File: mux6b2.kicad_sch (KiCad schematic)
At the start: 7 parts, among them U1 4081, U10 4071, U18 4069, U27 4069, U46 4071, U48 4081, U6 4081

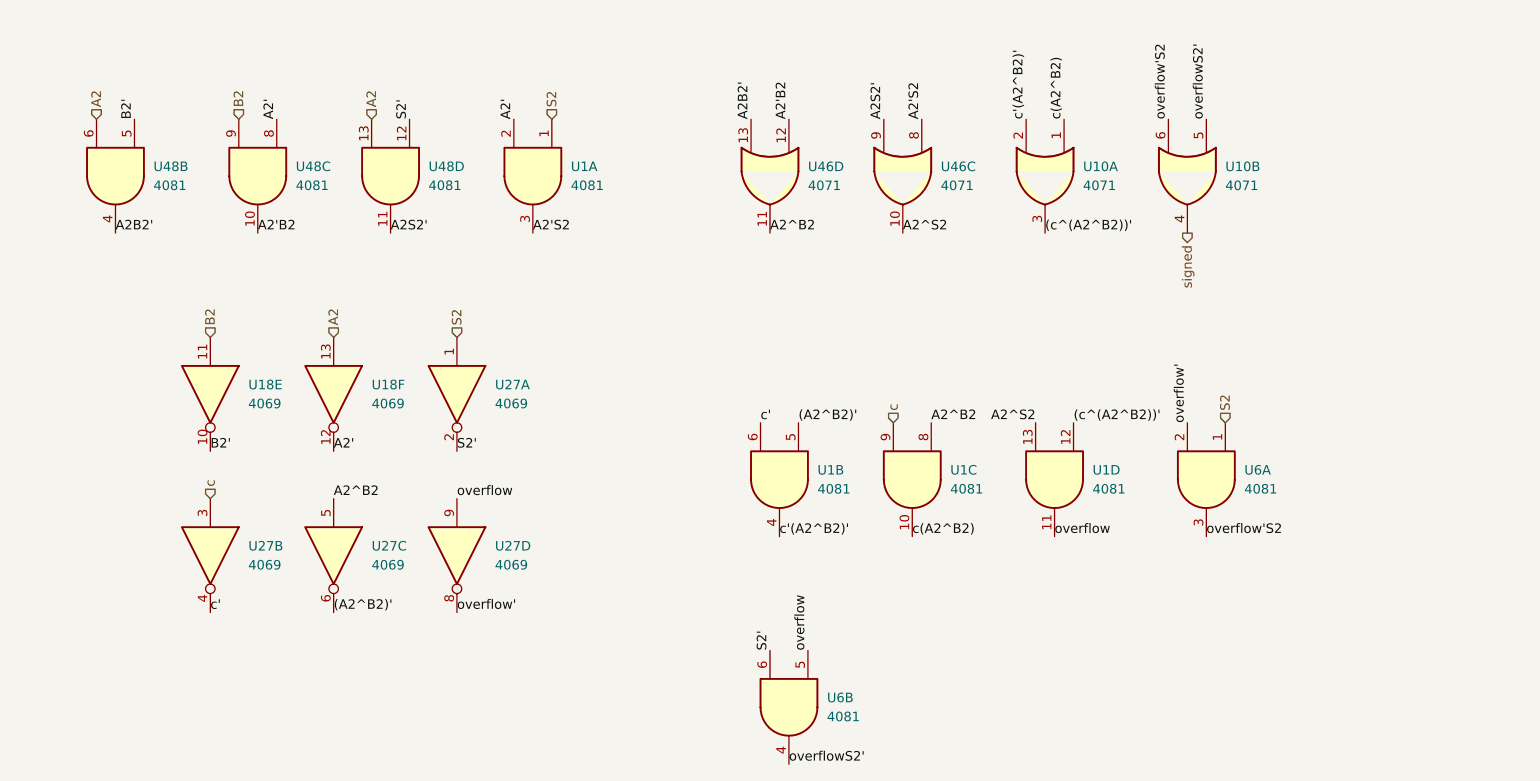
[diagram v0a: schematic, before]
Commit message: Add files via upload
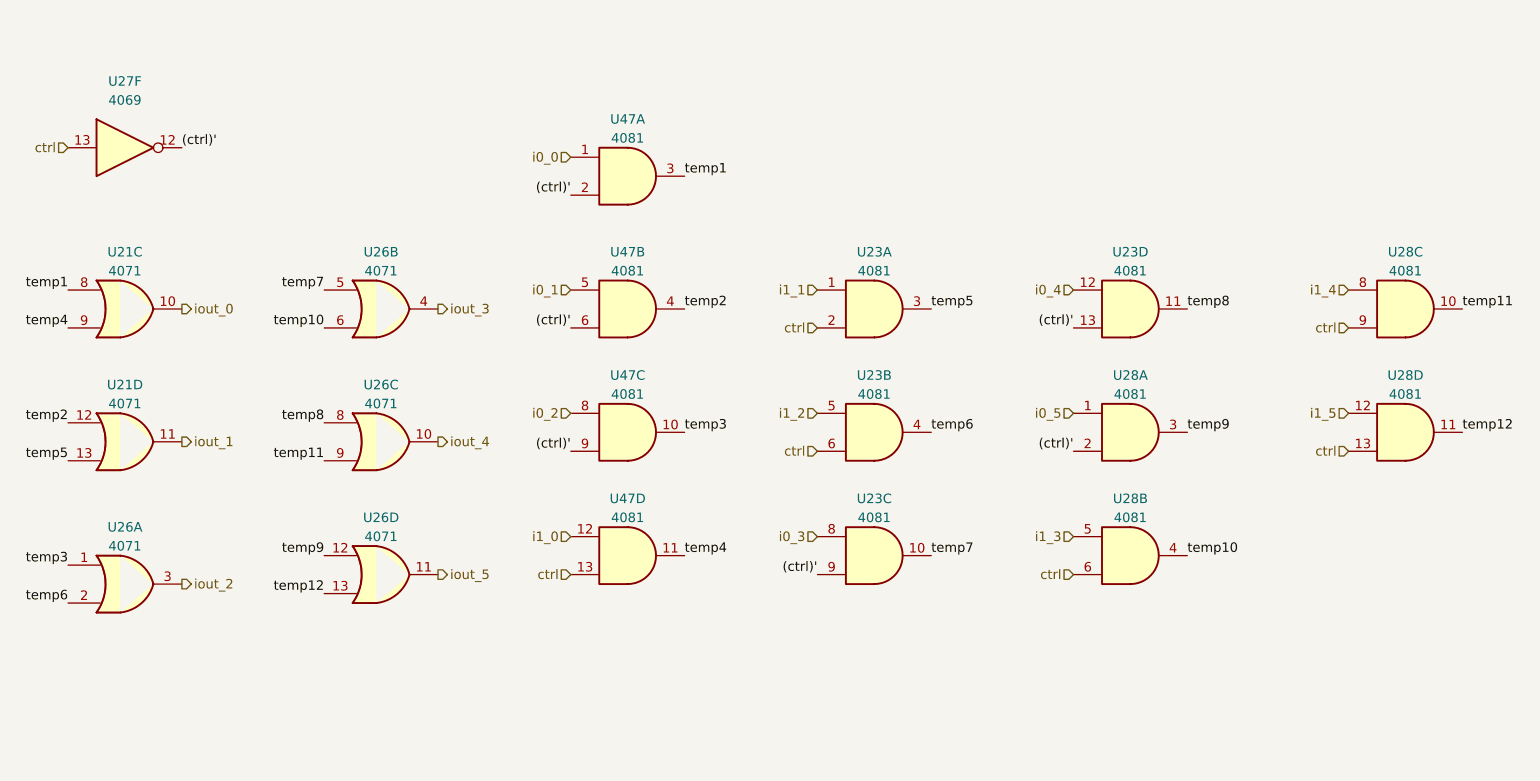
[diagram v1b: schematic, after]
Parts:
- removed U1, U48, U6: 4081, Package_DIP:CERDIP-14_W7.62mm_SideBrazed_LongPads_Socket, symbol 4xxx:4081
- removed U10, U46: 4071, Package_DIP:CERDIP-14_W7.62mm_SideBrazed_LongPads_Socket, symbol 4xxx:4071
- removed U18, U27: 4069, Package_DIP:CERDIP-14_W7.62mm_SideBrazed_LongPads_Socket, symbol 4xxx:4069
- added U21, U26: 4071, Package_DIP:CERDIP-14_W7.62mm_SideBrazed_LongPads_Socket, symbol 4xxx:4071
- added U23, U28, U47: 4081, Package_DIP:CERDIP-14_W7.62mm_SideBrazed_LongPads_Socket, symbol 4xxx:4081
- added U27: 4069, Package_DIP:CERDIP-14_W7.62mm_SideBrazed_LongPads_Socket, symbol 4xxx:4069
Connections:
- new net (ctrl)': U23.13, U23.9, U27.12, U28.2, U47.2, U47.6, U47.9
- new net ctrl: U23.2, U23.6, U27.13, U28.13, U28.6, U28.9, U47.13
- new net i0_0: U47.1
- new net i0_1: U47.5
- new net i0_2: U47.8
- new net i0_3: U23.8
- new net i0_4: U23.12
- new net i0_5: U28.1
- new net i1_0: U47.12
- new net i1_1: U23.1
- new net i1_2: U23.5
- new net i1_3: U28.5
- new net i1_4: U28.8
- new net i1_5: U28.12
- new net iout_0: U21.10
- new net iout_1: U21.11
- new net iout_2: U26.3
- new net iout_3: U26.4
- new net iout_4: U26.10
- new net iout_5: U26.11
- new net temp1: U21.8, U47.3
- new net temp10: U26.6, U28.4
- new net temp11: U26.9, U28.10
- new net temp12: U26.13, U28.11
- new net temp2: U21.12, U47.4
- new net temp3: U26.1, U47.10
- new net temp4: U21.9, U47.11
- new net temp5: U21.13, U23.3
- new net temp6: U23.4, U26.2
- new net temp7: U23.10, U26.5
- new net temp8: U23.11, U26.8
- new net temp9: U26.12, U28.3
